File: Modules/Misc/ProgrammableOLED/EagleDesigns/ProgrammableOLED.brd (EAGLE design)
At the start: 100 x 80 mm, 16 parts, among them U2 ATMEGA328P_TQFP

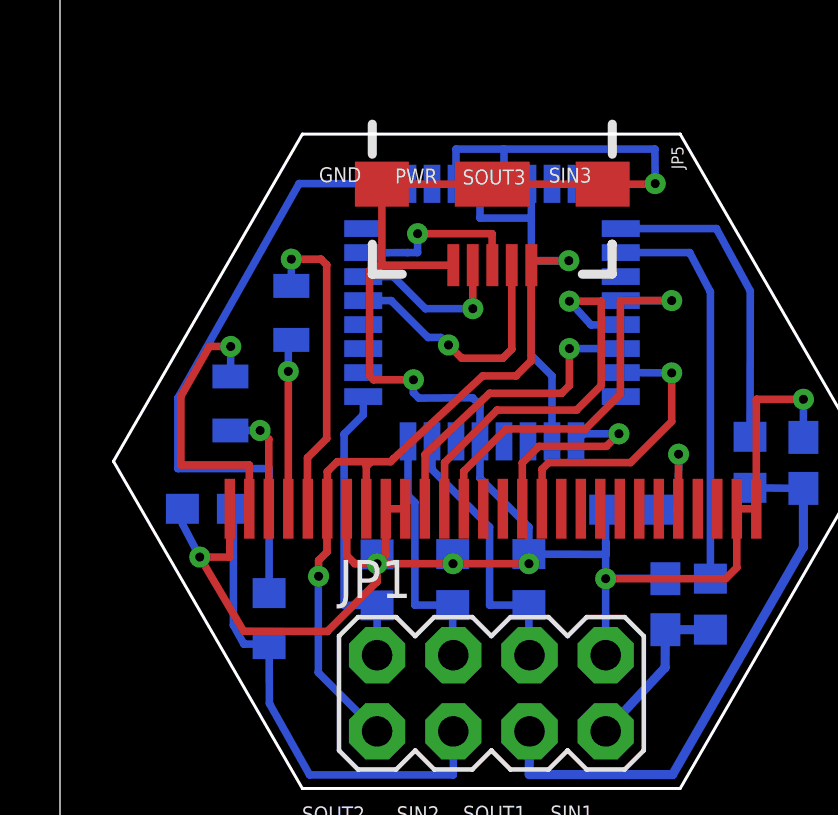
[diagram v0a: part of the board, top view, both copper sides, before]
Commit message: another round of minor fixes
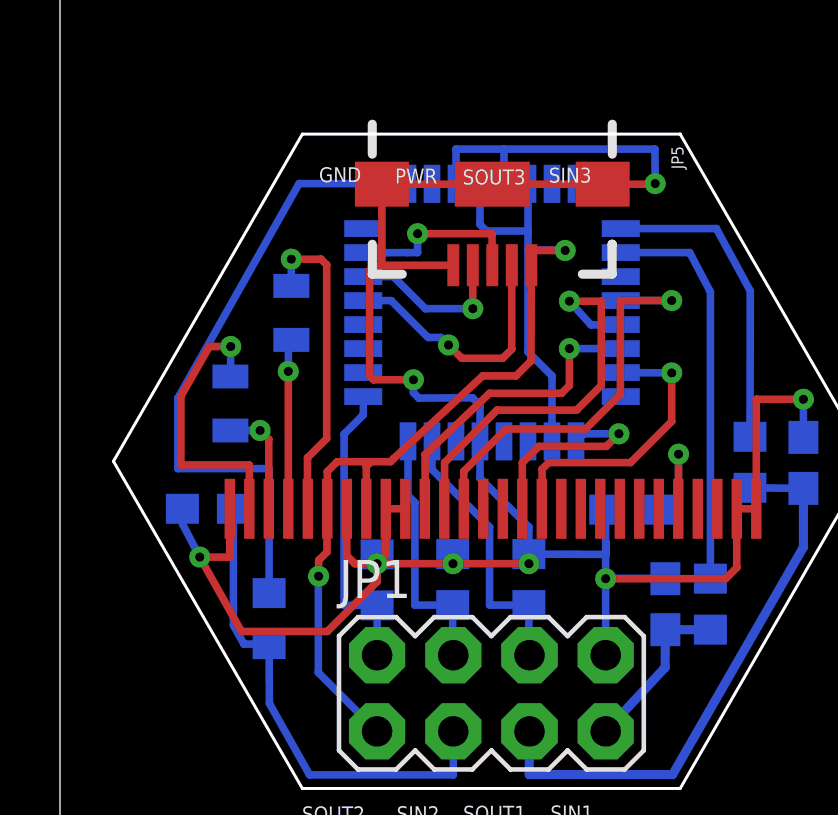
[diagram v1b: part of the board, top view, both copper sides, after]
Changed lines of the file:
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@@
 <layer number="21" name="tPlace" color="7" fill="1" visible="no" active="yes"/>
 <layer number="22" name="bPlace" color="7" fill="1" visible="no" active="yes"/>
-<layer number="23" name="tOrigins" color="15" fill="1" visible="yes" active="yes"/>
-<layer number="24" name="bOrigins" color="15" fill="1" visible="yes" active="yes"/>
+<layer number="23" name="tOrigins" color="15" fill="1" visible="no" active="yes"/>
+<layer number="24" name="bOrigins" color="15" fill="1" visible="no" active="yes"/>
 <layer number="25" name="tNames" color="7" fill="1" visible="no" active="yes"/>
 <layer number="26" name="bNames" color="7" fill="1" visible="no" active="yes"/>
@@
 <layer number="112" name="tSilk" color="7" fill="1" visible="no" active="yes"/>
 <layer number="113" name="IDFDebug" color="4" fill="1" visible="no" active="yes"/>
-<layer number="114" name="Badge_Outline" color="7" fill="1" visible="yes" active="yes"/>
-<layer number="115" name="ReferenceISLANDS" color="7" fill="1" visible="yes" active="yes"/>
+<layer number="114" name="Badge_Outline" color="7" fill="1" visible="no" active="yes"/>
+<layer number="115" name="ReferenceISLANDS" color="7" fill="1" visible="no" active="yes"/>
 <layer number="116" name="Patch_BOT" color="9" fill="4" visible="no" active="yes"/>
-<layer number="118" name="Rect_Pads" color="7" fill="1" visible="yes" active="yes"/>
+<layer number="118" name="Rect_Pads" color="7" fill="1" visible="no" active="yes"/>
 <layer number="121" name="_tsilk" color="7" fill="1" visible="no" active="yes"/>
 <layer number="122" name="_bsilk" color="7" fill="1" visible="no" active="yes"/>
@@
 <layer number="127" name="_tValues" color="7" fill="1" visible="no" active="yes"/>
 <layer number="128" name="_bValues" color="7" fill="1" visible="no" active="yes"/>
-<layer number="129" name="Mask" color="7" fill="1" visible="yes" active="yes"/>
+<layer number="129" name="Mask" color="7" fill="1" visible="no" active="yes"/>
 <layer number="131" name="tAdjust" color="7" fill="1" visible="no" active="yes"/>
 <layer number="132" name="bAdjust" color="7" fill="1" visible="no" active="yes"/>
@@
 <wire x1="23.22" y1="15.17" x2="23.21" y2="15.16" width="0.254" layer="1"/>
 <wire x1="23.21" y1="15.16" x2="23.21" y2="11.52" width="0.254" layer="1"/>
-<wire x1="8.91" y1="7.43" x2="6.12" y2="7.44" width="0.254" layer="1"/>
-<wire x1="6.12" y1="7.44" x2="4.66" y2="9.91" width="0.254" layer="1"/>
+<wire x1="8.91" y1="7.43" x2="6.05" y2="7.43" width="0.254" layer="1"/>
+<wire x1="6.05" y1="7.43" x2="4.66" y2="9.91" width="0.254" layer="1"/>
 <via x="4.66" y="9.91" extent="1-16" drill="0.3" diameter="0.254"/>
 <wire x1="4.08" y1="11.52" x2="4.08" y2="11.02" width="0.254" layer="16"/>
@@
 <contactref element="JP5" pad="VBUS1"/>
 <wire x1="16.4" y1="13.7674" x2="16.42" y2="13.7874" width="0.254" layer="16"/>
-<wire x1="15.6" y1="22.3526" x2="15.69" y2="22.2626" width="0.254" layer="16"/>
 <wire x1="10.57" y1="4.1" x2="8.61" y2="6.06" width="0.254" layer="16"/>
 <wire x1="8.61" y1="6.06" x2="8.61" y2="9.26" width="0.254" layer="16"/>
@@
 <wire x1="15.2" y1="15.95" x2="15.7" y2="16.45" width="0.254" layer="1"/>
 <wire x1="15.7" y1="16.45" x2="15.71" y2="19.64" width="0.254" layer="1"/>
-<wire x1="15.71" y1="19.79" x2="15.71" y2="19.64" width="0.254" layer="1"/>
 <wire x1="16.4" y1="13.7674" x2="16.4" y2="15.95" width="0.254" layer="16"/>
-<wire x1="16.4" y1="15.95" x2="15.71" y2="16.64" width="0.254" layer="16"/>
-<wire x1="15.71" y1="21.18" x2="15.71" y2="22.2426" width="0.254" layer="16"/>
-<wire x1="15.71" y1="22.2426" x2="15.6" y2="22.3526" width="0.254" layer="16"/>
-<wire x1="14" y1="22.3526" x2="14" y2="21.22" width="0.254" layer="16"/>
-<wire x1="14" y1="21.22" x2="14.01" y2="21.21" width="0.254" layer="16"/>
-<wire x1="14.01" y1="21.21" x2="15.68" y2="21.21" width="0.254" layer="16"/>
-<wire x1="15.68" y1="21.21" x2="15.71" y2="21.18" width="0.254" layer="16"/>
-<wire x1="15.71" y1="21.18" x2="15.71" y2="19.79" width="0.254" layer="16"/>
-<wire x1="15.71" y1="19.79" x2="16.96" y2="19.79" width="0.254" layer="16"/>
-<via x="16.96" y="19.79" extent="1-16" drill="0.3"/>
-<wire x1="16.96" y1="19.79" x2="15.71" y2="19.79" width="0.254" layer="1"/>
-<wire x1="15.71" y1="16.64" x2="15.71" y2="19.79" width="0.254" layer="16"/>
 <wire x1="9.24" y1="13.09" x2="10.37" y2="13.09" width="0.254" layer="1"/>
 <wire x1="10.37" y1="13.09" x2="11.02" y2="13.09" width="0.254" layer="1"/>
 <wire x1="11.02" y1="13.09" x2="11.125" y2="13.195" width="0.254" layer="1"/>
 <wire x1="10.21" y1="12.93" x2="10.37" y2="13.09" width="0.254" layer="1"/>
+<wire x1="15.6" y1="22.3526" x2="15.6" y2="20.77" width="0.254" layer="16"/>
+<wire x1="15.6" y1="20.77" x2="15.6" y2="20.14" width="0.254" layer="16"/>
+<wire x1="15.6" y1="16.75" x2="16.4" y2="15.95" width="0.254" layer="16"/>
+<wire x1="14" y1="22.3526" x2="14" y2="21" width="0.254" layer="16"/>
+<wire x1="14" y1="21" x2="14.22" y2="20.78" width="0.254" layer="16"/>
+<wire x1="14.22" y1="20.78" x2="15.59" y2="20.78" width="0.254" layer="16"/>
+<wire x1="15.59" y1="20.78" x2="15.6" y2="20.77" width="0.254" layer="16"/>
+<wire x1="15.6" y1="16.75" x2="15.6" y2="20.14" width="0.254" layer="16"/>
+<wire x1="15.6" y1="20.14" x2="16.83" y2="20.14" width="0.254" layer="16"/>
+<wire x1="16.83" y1="20.14" x2="16.84" y2="20.13" width="0.254" layer="16"/>
+<via x="16.84" y="20.13" extent="1-16" drill="0.3"/>
+<wire x1="16.84" y1="20.13" x2="15.78" y2="20.13" width="0.254" layer="1"/>
+<wire x1="15.78" y1="20.13" x2="15.75" y2="20.16" width="0.254" layer="1"/>
+<wire x1="15.75" y1="20.16" x2="15.75" y2="19.68" width="0.254" layer="1"/>
+<wire x1="15.75" y1="19.68" x2="15.71" y2="19.64" width="0.254" layer="1"/>
 </signal>
 <signal name="RESET">
